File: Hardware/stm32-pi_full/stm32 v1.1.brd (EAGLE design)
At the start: 131.4 x 105.8 mm, 272 parts, among them J1 JUMPER-SMT_2_NC_TRACE_NO-SILK, Q1 PNP, Q2 NPN, Q3 NPN, U1 ESP32-WROOM-32D, U2 RFM69HCW/RFM95W

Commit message: sync
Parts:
- added C57, C59, C60: 22uF, rcl:C0805
- added C58, C61: 100nF, resistor:C0603
- FB1: value 1600R -> 600R
- FB10, FB11, FB5: value (none) -> 0R
- FB6: value (none) -> 600R
- R22: value 0R -> (none)
- moved C56 317.6 mm to (120.8, 81.2)
- moved C36 291.6 mm to (101.0, 77.4)
- moved C50 286.5 mm to (74.0, 79.5), turned to 90 degrees
- moved D8 282.3 mm to (72.1, 95.9)
- moved LED_PWR 282.2 mm to (121.9, 36.2), turned to 180 degrees
- moved D11 281.5 mm to (10.9, 65.2)
- moved C49 281.0 mm to (51.9, 49.1)
- moved D7 278.8 mm to (70.4, 95.9), turned to 180 degrees
- moved D9 275.6 mm to (32.3, 95.9), turned to 180 degrees
- moved D3 274.0 mm to (12.7, 60.7), turned to 180 degrees
- moved D10 272.9 mm to (33.9, 95.9)
- moved C35 268.2 mm to (45.9, 80.5), turned to 90 degrees
- moved D2 251.4 mm to (88.4, 10.4)
- moved C53 227.3 mm to (15.3, 20.1), flipped to the bottom
- moved D5 224.6 mm to (108.3, 95.7), turned to 180 degrees
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- renumbered RB10 to R60, RB11 to R63, RB12 to R64, RB13 to R65, RB14 to R61, RB15 to R62, RB16 to R66, RB17 to R67, RB18 to R68
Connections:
- net +5V: no longer TB2.P$6, U$2.IN+, U$2.IN+1
- net +5V_USB: now also C58.1, C59.1, C60.1, TB2.P$6, U$2.IN+, U$2.IN+1
- net AGND: now also C57.2, C61.2
- net DGND: now also C58.2, C59.2, C60.2
- net N$29: now also C57.1, C61.1
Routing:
- net +5V_USB: track 14.4 -> 65.5 mm, vias 0 -> 1
- net +5V: track 305.1 -> 269.4 mm, vias 3 -> 2
- net +3V3: track 79.2 -> 94.8 mm, vias 25 -> 27
- net 3PH_BIAS: track 66.6 -> 80.2 mm
- net STM32_OPAMP_OUT: track 16.0 -> 4.68 mm, vias 1 -> 0
- net EXT_TERM2: track 58.9 -> 66.6 mm
- net +3V3ANA: track 30.4 -> 37.1 mm, vias 20 -> 21
- net BOOT_STM: track 160.8 -> 167.5 mm
- net SD_CS: track 41.7 -> 47.9 mm
- net BIAS123: track 72.0 -> 77.9 mm
- net BIAS456: track 68.1 -> 74.0 mm
- net EXT_TERM1: track 62.0 -> 67.9 mm
- net BIAS789: track 61.8 -> 67.7 mm
- net BIAS_INPUT: track 129.1 -> 134.0 mm
- net N$29: track 9.79 -> 14.4 mm
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
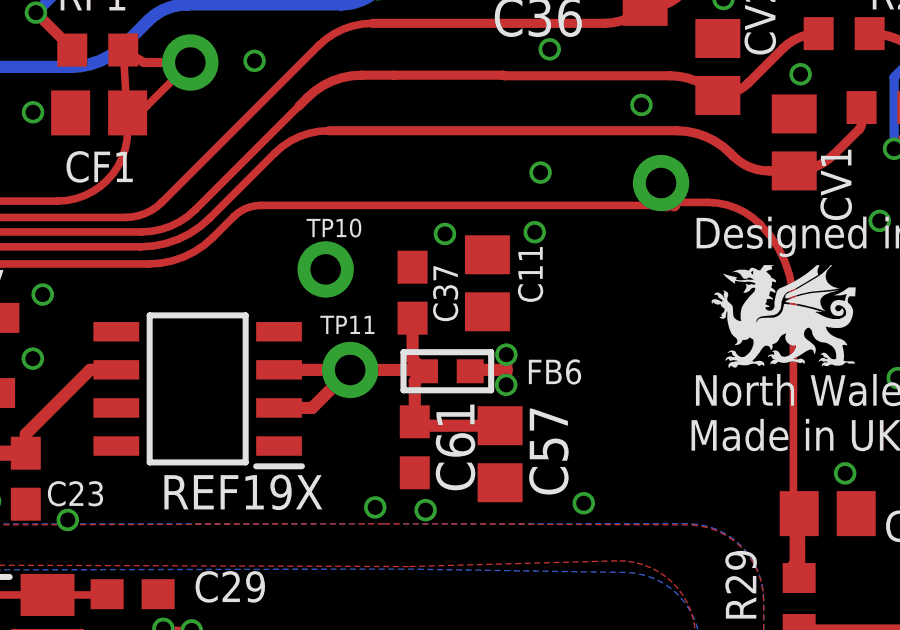
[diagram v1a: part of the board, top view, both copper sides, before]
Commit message: modified:   Hardware/stm32-pi_basic/6/stm32hw06.brd 	modified:   Hardware/stm32-pi_full/stm32 v1.1.brd 	deleted:    Protecting Inputs in Digital Electronics ESD Protection | DigiKey.pdf
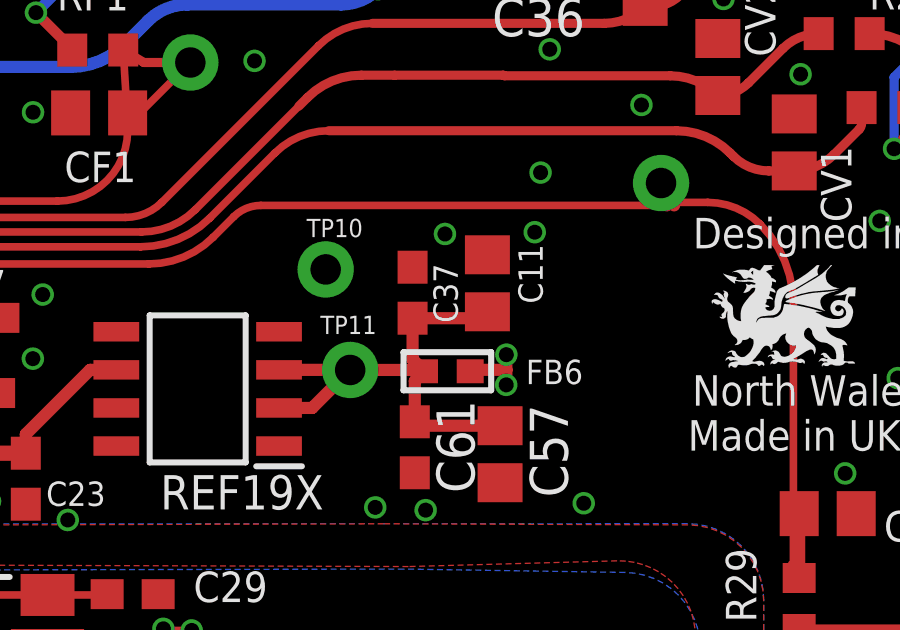
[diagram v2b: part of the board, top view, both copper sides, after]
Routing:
- net GND_USB: track 3.56 -> 7.74 mm
- net N$29: track 14.4 -> 17.0 mm
